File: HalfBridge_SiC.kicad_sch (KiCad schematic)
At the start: 4 parts, among them J4 Screw_Terminal_01x02, SW2 CAS-D20X1

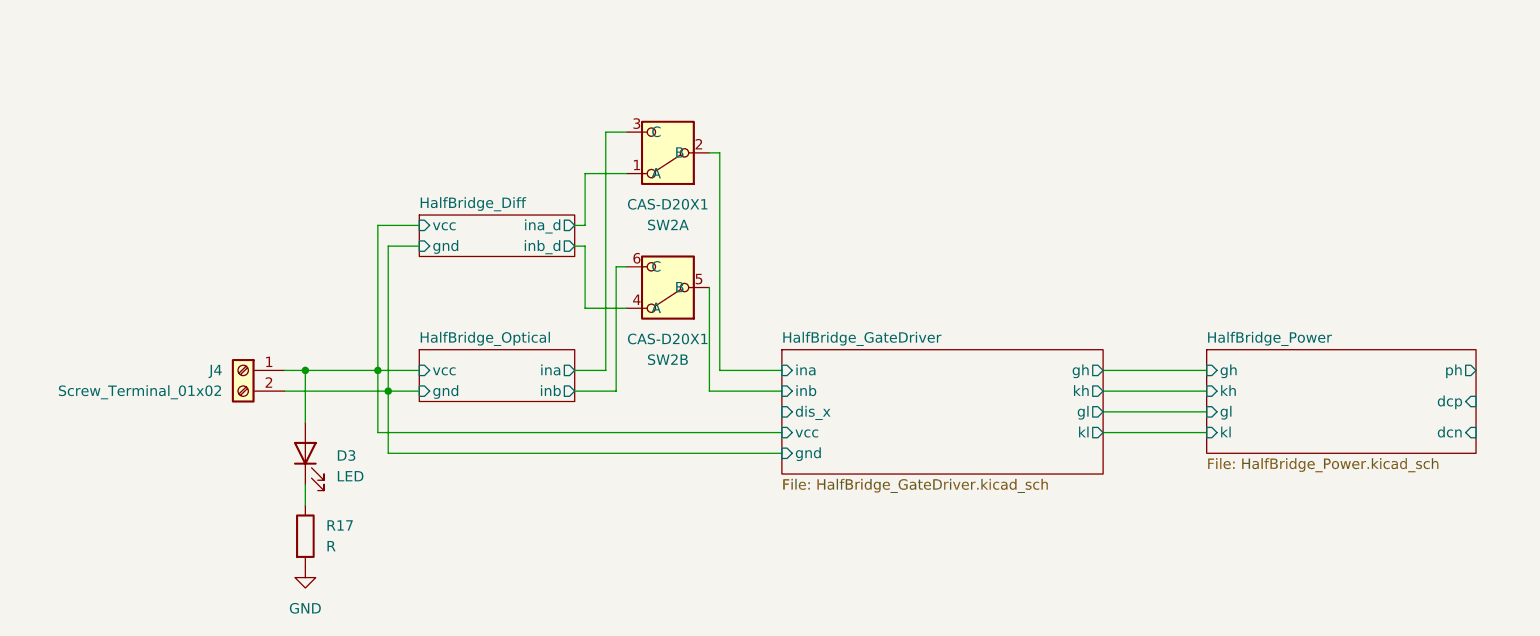
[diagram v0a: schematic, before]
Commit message: new optical diff xor
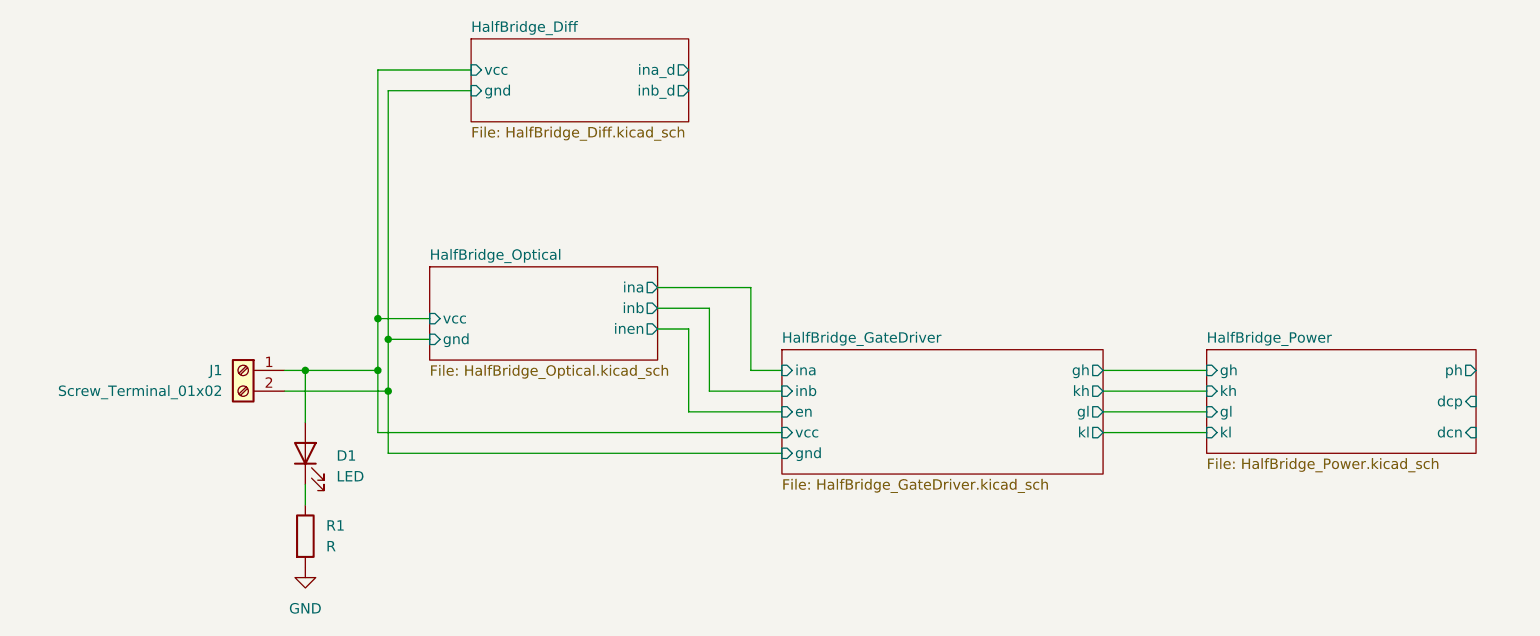
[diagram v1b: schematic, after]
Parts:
- removed SW2: CAS-D20X1, My_Button_Switch_SMD:Nidec_Copal_CAS-D20A1, symbol My_Switch:CAS-D20X1
- renumbered D3 to D1, J4 to J1, R17 to R1
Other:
- sheet HalfBridge_GateDriver ports: added en; removed dis_x
- sheet HalfBridge_Optical ports: added inen; removed none
